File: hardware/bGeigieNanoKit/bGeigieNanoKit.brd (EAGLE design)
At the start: 104.8 x 66.7 mm, 36 parts, among them T1 2SC1815

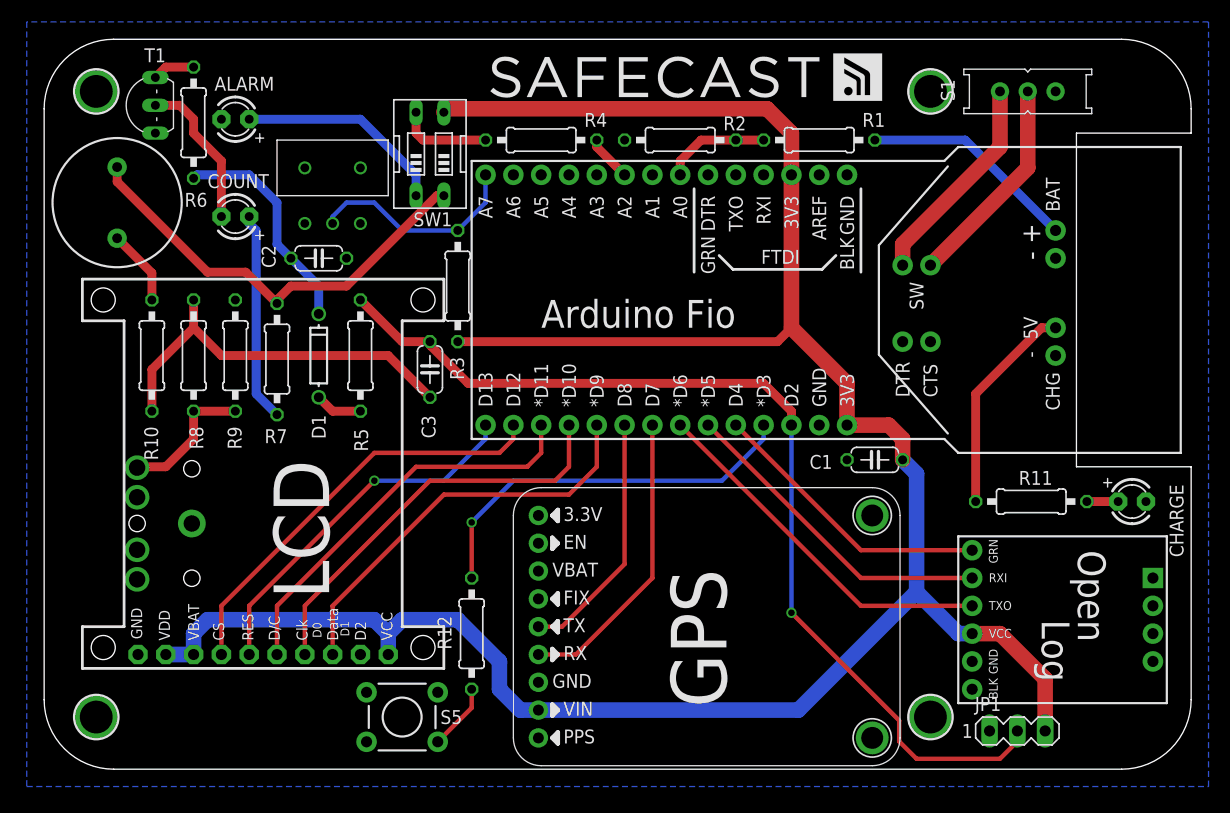
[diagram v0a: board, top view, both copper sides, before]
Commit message: rc1
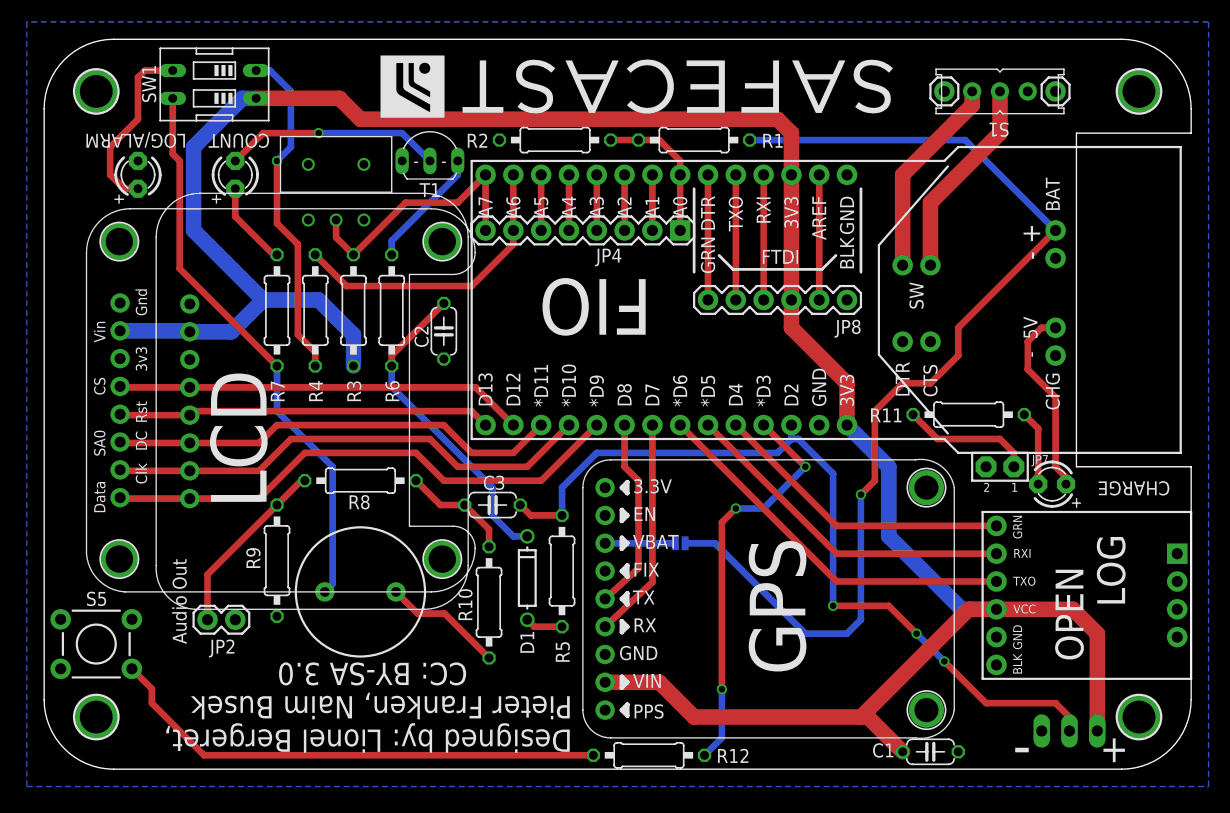
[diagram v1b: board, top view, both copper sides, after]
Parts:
- removed ALARM: RED, adafruit:LED3MM
- removed CN1: (no value), microbuilder:STX3100
- removed U$1: OPENLOG, open_hw_sockets:OPENLOG
- removed U$10: (no value), open_hw_sockets:SAFECAST_LOGO1
- removed U$3: GPS, open_hw_sockets:ULTIMATE_GPS_V3_TOP
- added GPS: ULTIMATE_GPSTOP, open_hw_sockets:ULTIMATE_GPS_V3_TOP
- added JP2: (no value), SparkFun:1X02
- added JP3, JP5: M01PTH, SparkFun:1X01
- added JP4: (no value), SparkFun:1X08
- added JP6: (no value), SparkFun:SJ_2S-NO
- added JP7: (no value), microbuilder:JUMPER2
- added JP8: (no value), SparkFun:1X06
- added LCD: SSD1306_128X64_V2_LCD1.3IN_TOP, open_hw_sockets:SSD1306_128X64_1.3IN_LCD_TOP
- added LCD2: SSD1306_128X64_V2_LCD0.96IN_MIN, open_hw_sockets:SSD1306_128X64_0.96IN_MIN_LCD
- added LOG/ALARM: RED, adafruit:LED3MM
- added OPENLOG: OPENLOG, open_hw_sockets:OPENLOG
- JP1: device con-lstb:MA03-1 -> pinhead:1X03/90
- U$5: value LCD -> (none); device open_hw_sockets:SSD1306_128X64_LCD_MIN -> open_hw_sockets:SAFECAST_LOGO2
- moved U$5 72.5 mm to (79.7, 67.3), turned to 180 degrees
- moved SG1 41.9 mm to (30.5, 17.8), turned to 180 degrees
- moved R10 38.2 mm to (42.2, 16.8), turned to 90 degrees
- moved S5 28.7 mm to (6.35, 13.0)
- moved D1 27.9 mm to (45.7, 19.1)
- moved C1 27.1 mm to (82.5, 3.17), turned to 180 degrees
- moved R5 27.0 mm to (48.9, 19.7)
- moved R4 25.8 mm to (26.4, 43.5), turned to 270 degrees
- moved T1 25.6 mm to (36.8, 57.1), turned to 0 degrees
- moved R6 24.9 mm to (33.3, 43.5)
- moved SW1 20.7 mm to (17.1, 64.1), turned to 90 degrees
- moved R12 19.6 mm to (56.8, 2.86), turned to 0 degrees
- moved R9 19.1 mm to (22.9, 20.6), turned to 270 degrees
- moved R8 19.0 mm to (30.5, 27.9), turned to 0 degrees
- moved U$6 19.0 mm to (101.6, 63.5)
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- renumbered U$2 to FIO
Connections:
- removed net VBAT: U$3.JP1$7
- new net N$31: CHARGE.K, R11.2
- new net N$32: R7.1, SG1.+, SW1.4
- new net N$33: FIO.JP5$11, JP4.5
- new net N$34: FIO.JP5$10, JP4.4
- new net N$35: FIO.JP5$9, JP4.3
- new net N$36: FIO.JP5$8, JP4.2
- new net N$37: FIO.JP5$6, JP8.6
- new net N$38: FIO.JP5$5, JP8.5
- new net N$39: FIO.JP5$4, JP8.4
- new net N$40: FIO.JP5$2, JP8.2
- new net VGPS: GPS.JP1$7, JP6.2
- net GND: now also GPS.JP1$3, GPS.U$8$P$1, GPS.U$9$P$1, JP1.3, JP2.2, JP7.2, JP8.1, LCD.JP1$8, LCD.U$23$P$1, LCD.U$24$P$1, LCD.U$25$P$1, LCD.U$26$P$1, LCD2.JP1$8, LOG/ALARM.K, OPENLOG.JP1$5, OPENLOG.JP1$6, U$4.P$1; no longer ALARM.K, CHARGE.K, CN1.1, JP1.1, U$1.JP1$5, U$1.JP1$6, U$3.JP1$3, U$3.U$8$P$1, U$3.U$9$P$1, U$4.P$3, U$5.P0\$10
- net N$1: now also LCD.JP1$1, LCD2.JP1$1; no longer U$5.P0\$3
- net N$10: now also OPENLOG.JP1$1; no longer U$1.JP1$1
- net N$11: now also JP4.1
- net N$14: now also JP4.8
- net N$15: now also FIO.JP5$13, JP4.7; no longer FIO.JP5$9
- net N$16: now also LOG/ALARM.A, SW1.3; no longer ALARM.A, SW1.1
- net N$17: now also SW1.2; no longer SW1.4
- net N$2: now also LCD.JP1$2, LCD2.JP1$2; no longer U$5.P0\$4
- net N$21: now also FIO.JP5$12, JP4.6; no longer R7.1, SG1.+, SW1.2
- net N$25: now also JP2.1; no longer CN1.2
- net N$29: now also JP7.1; no longer CHARGE.A
- net N$3: now also LCD.JP1$3, LCD2.JP1$3; no longer U$5.P0\$5
- net N$4: now also LCD.JP1$5, LCD2.JP1$5; no longer U$5.P0\$7
- net N$5: now also LCD.JP1$4, LCD2.JP1$4; no longer U$5.P0\$6
- net N$6: now also GPS.JP1$5; no longer U$3.JP1$5
- net N$7: now also GPS.JP1$4; no longer U$3.JP1$4
- net N$8: now also OPENLOG.JP1$3; no longer U$1.JP1$3
- net N$9: now also OPENLOG.JP1$2; no longer U$1.JP1$2
- net VBATT: now also JP6.1
- net VCC: now also GPS.JP1$2, JP1.1, JP8.3, LCD.JP1$7, LCD2.JP1$7, OPENLOG.JP1$4, SW1.1; no longer JP1.3, SW1.3, U$1.JP1$4, U$3.JP1$2, U$5.P0\$1, U$5.P0\$8, U$5.P0\$9
- net VIN: now also CHARGE.A; no longer R11.2
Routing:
- net VBATT: track 19.9 -> 95.8 mm, vias 0 -> 1
- net N$32: track 0.00 -> 51.4 mm
- net N$20: track 6.08 -> 46.2 mm
- net N$21: track 40.1 -> 5.08 mm
- net N$24: track 36.0 -> 10.1 mm
- net N$15: track 4.23 -> 27.2 mm
- net N$17: track 8.52 -> 31.0 mm, vias 0 -> 1
- net N$18: track 91.1 -> 75.1 mm, vias 1 -> 3
- net N$40: track 0.00 -> 11.4 mm
- net N$39: track 0.00 -> 11.4 mm
- net N$38: track 0.00 -> 11.4 mm
- net N$37: track 0.00 -> 11.4 mm
- net N$19: track 19.1 -> 7.80 mm
- net N$1: track 37.6 -> 48.4 mm
- net N$29: track 2.86 -> 11.9 mm
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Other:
- board text added: "+"
- board text added: "-"
- board text added: "Audio Out"
- board text added: "Designed by: Lionel Bergeret, Pieter Franken, Naim Busek CC: BY-SA 3.0"
- board text added: "FIO"
- board text added: "GPS"
- board text added: "LCD"
- board text added: "OPEN LOG"
- board text added: "Special thanks to: Joe, Rob, Jurgen, Sean, Robin, Akiba, Shigeru, Joi, Dan, Medcom, Loftwork, FabCafe, Tokyo Hacker Space, CRASH Space, Adafruit, Sparkfun, Pelican"
